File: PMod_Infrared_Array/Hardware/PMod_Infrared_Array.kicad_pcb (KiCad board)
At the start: 2 copper layers, 50 x 18 mm, 17 parts, among them IC1 AMG8834, J1 Conn_02x06_Counter_Clockwise

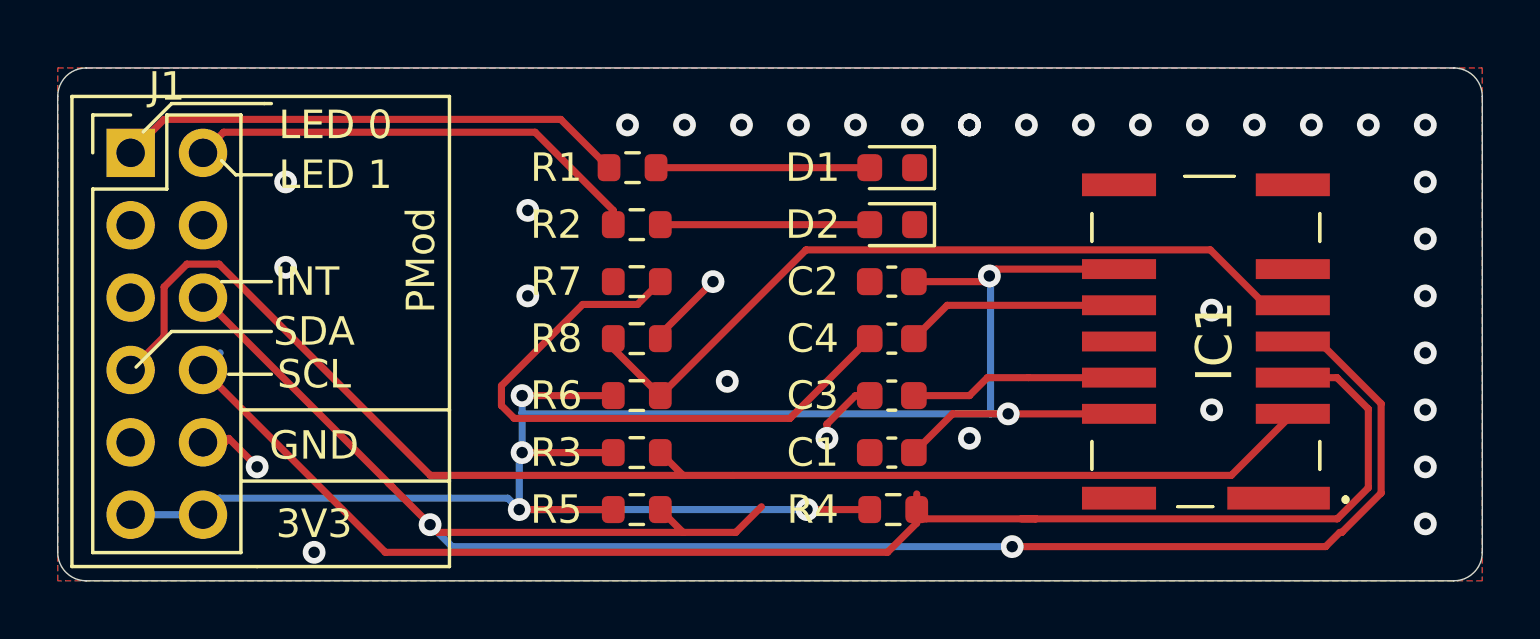
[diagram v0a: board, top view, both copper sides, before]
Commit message: change the workflow runs reasons
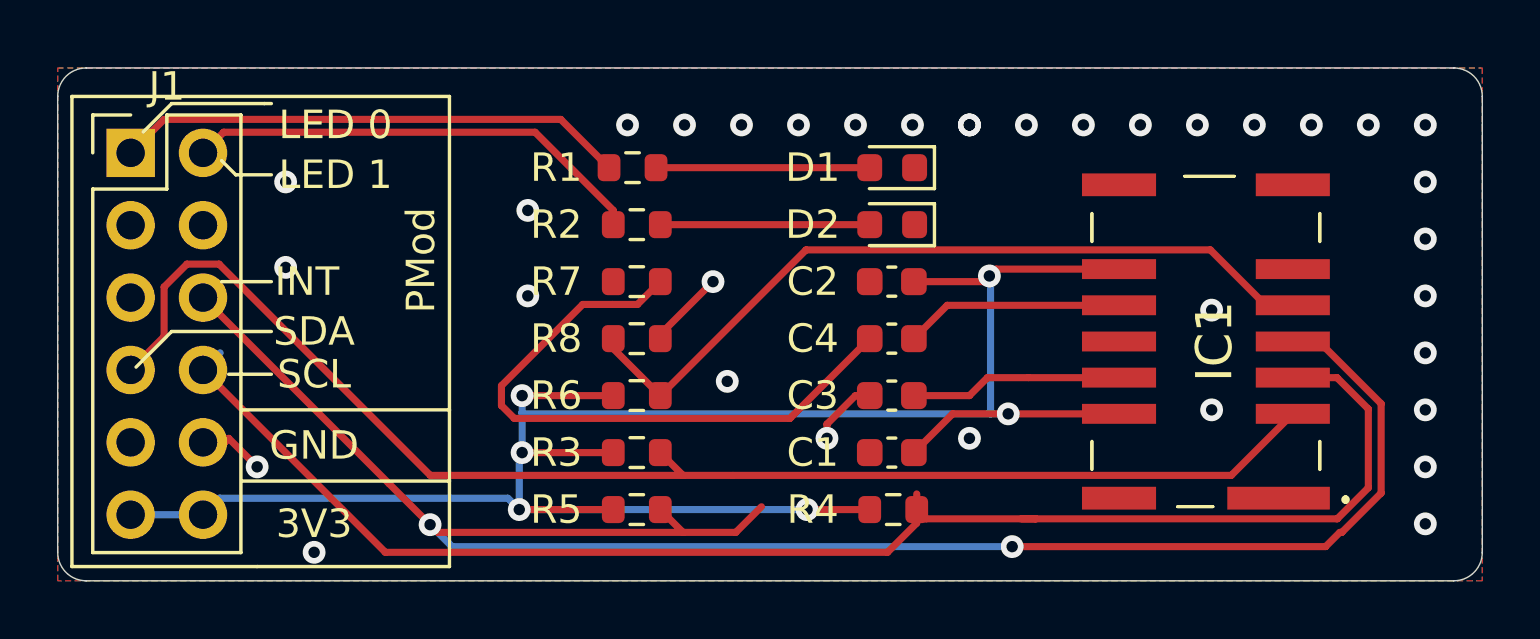
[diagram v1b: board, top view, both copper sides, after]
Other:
- net class Default removed

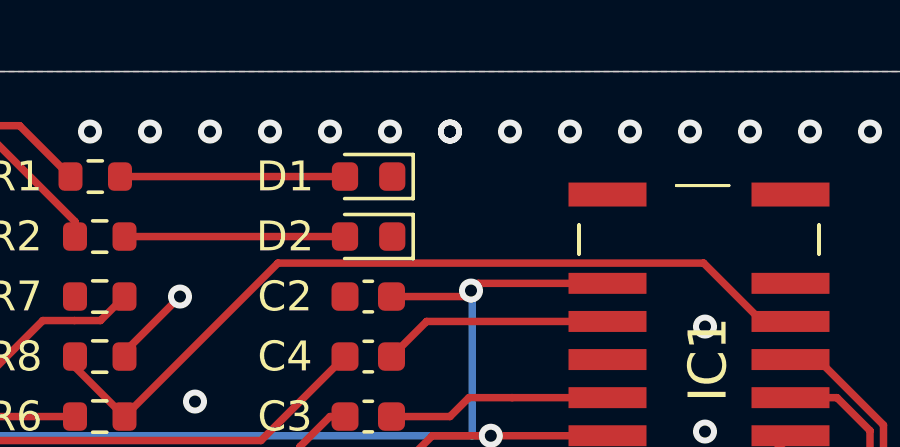
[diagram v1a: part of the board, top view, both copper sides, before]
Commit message: fix some pcb errors
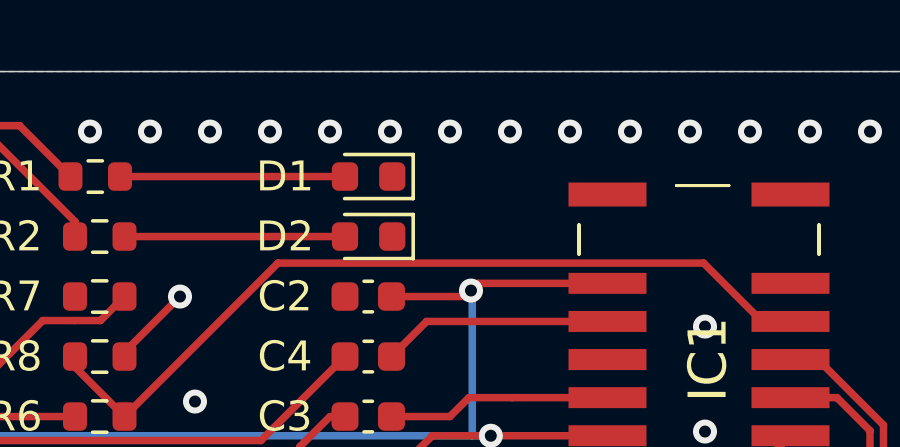
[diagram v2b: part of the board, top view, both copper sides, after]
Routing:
- net GND: vias 35 -> 34
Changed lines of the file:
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@@
   (via (at 150.5 88) (size 0.8) (drill 0.4) (layers "F.Cu" "B.Cu") (net 1))
   (via (at 158 86) (size 0.8) (drill 0.4) (layers "F.Cu" "B.Cu") (net 1))
-  (via (at 142 78) (size 0.8) (drill 0.4) (layers "F.Cu" "B.Cu") (net 1))
   (via (at 142 89) (size 0.8) (drill 0.4) (layers "F.Cu" "B.Cu") (net 1))
   (via (at 150.5 84.5) (size 0.8) (drill 0.4) (layers "F.Cu" "B.Cu") (net 1))

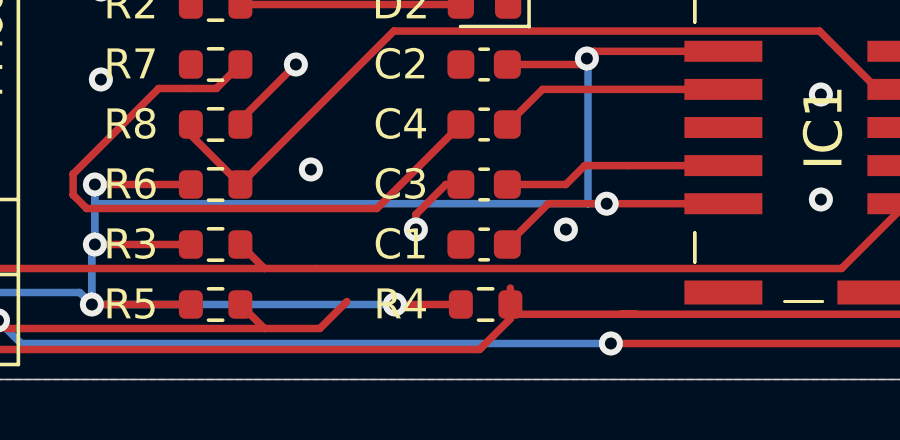
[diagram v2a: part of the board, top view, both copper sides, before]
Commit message: design rule fixes
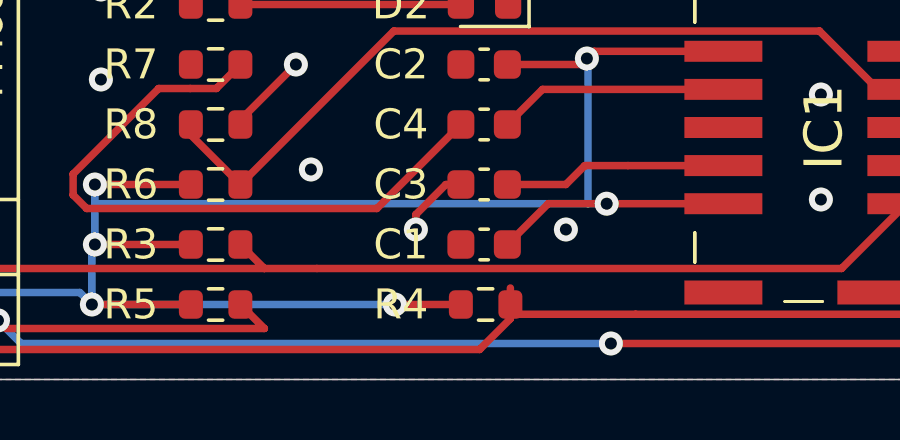
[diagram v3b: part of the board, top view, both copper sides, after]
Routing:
- net INT: track 66.1 -> 63.0 mm
- net SCL: track 52.8 -> 52.3 mm
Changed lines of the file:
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@@
   (segment (start 154.50002 92.8) (end 143.5 92.8) (width 0.25) (layer "F.Cu") (net 13))
   (segment (start 156.450009 87.783599) (end 154.26641 85.6) (width 0.25) (layer "F.Cu") (net 13))
-  (segment (start 131.95001 92.30001) (end 133.80001 92.30001) (width 0.25) (layer "F.Cu") (net 13))
   (segment (start 121.62 90.58) (end 123.07 92.03) (width 0.25) (layer "F.Cu") (net 13))
   (segment (start 121.62 90.58) (end 115.1 84.06) (width 0.25) (layer "F.Cu") (net 13))
   (segment (start 156.45001 90.921402) (end 156.450009 87.783599) (width 0.25) (layer "F.Cu") (net 13))
   (segment (start 154.26641 85.6) (end 153.35 85.6) (width 0.25) (layer "F.Cu") (net 13))
-  (segment (start 133.80001 92.30001) (end 134.7 91.40002) (width 0.25) (layer "F.Cu") (net 13))
   (segment (start 155.071402 92.30001) (end 155.00001 92.30001) (width 0.25) (layer "F.Cu") (net 13))
   (via (at 123.07 92.03) (size 0.8) (drill 0.4) (layers "F.Cu" "B.Cu") (net 13))
@@
   (segment (start 143.5 92.8) (end 123.84 92.8) (width 0.25) (layer "B.Cu") (net 13))
   (segment (start 123.84 92.8) (end 123.07 92.03) (width 0.25) (layer "B.Cu") (net 13))
-  (segment (start 144.325001 91.825001) (end 143.825001 91.825001) (width 0.25) (layer "F.Cu") (net 14))
   (segment (start 156 87.97) (end 154.9 86.87) (width 0.25) (layer "F.Cu") (net 14))
   (segment (start 154.9 86.87) (end 153.35 86.87) (width 0.25) (layer "F.Cu") (net 14))
